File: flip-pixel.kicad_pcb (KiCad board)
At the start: 2 copper layers, 157.5 x 129.5 mm, 183 parts, among them J1 Barrel-Jack, Q1 DMN62D0U-7, Q10 STS8DN6LF6AG, Q11 DMN62D0U-7, Q12 DMN62D0U-7, Q13 STS8DN6LF6AG, Q14 DMN62D0U-7, Q15 DMN62D0U-7, Q16 STS8DN6LF6AG, Q17 DMN62D0U-7, Q18 DMN62D0U-7, Q19 STS8DN6LF6AG, Q2 DMN62D0U-7, Q20 DMN62D0U-7, Q21 DMN62D0U-7, Q22 STS8DN6LF6AG, Q23 DMN62D0U-7, Q24 DMN62D0U-7, Q25 STS8DN6LF6AG, Q26 DMN62D0U-7, Q27 DMN62D0U-7, Q28 STS8DN6LF6AG, Q29 DMN62D0U-7, Q3 DMN62D0U-7, Q30 DMN62D0U-7, Q31 STS8DN6LF6AG, Q4 STS8DN6LF6AG, Q5 DMN62D0U-7, Q6 DMN62D0U-7, Q7 STS8DN6LF6AG, Q8 DMN62D0U-7, Q9 DMN62D0U-7, U1 LM2665M6, U2 ESP32_DevBoard, U3 INA250A3

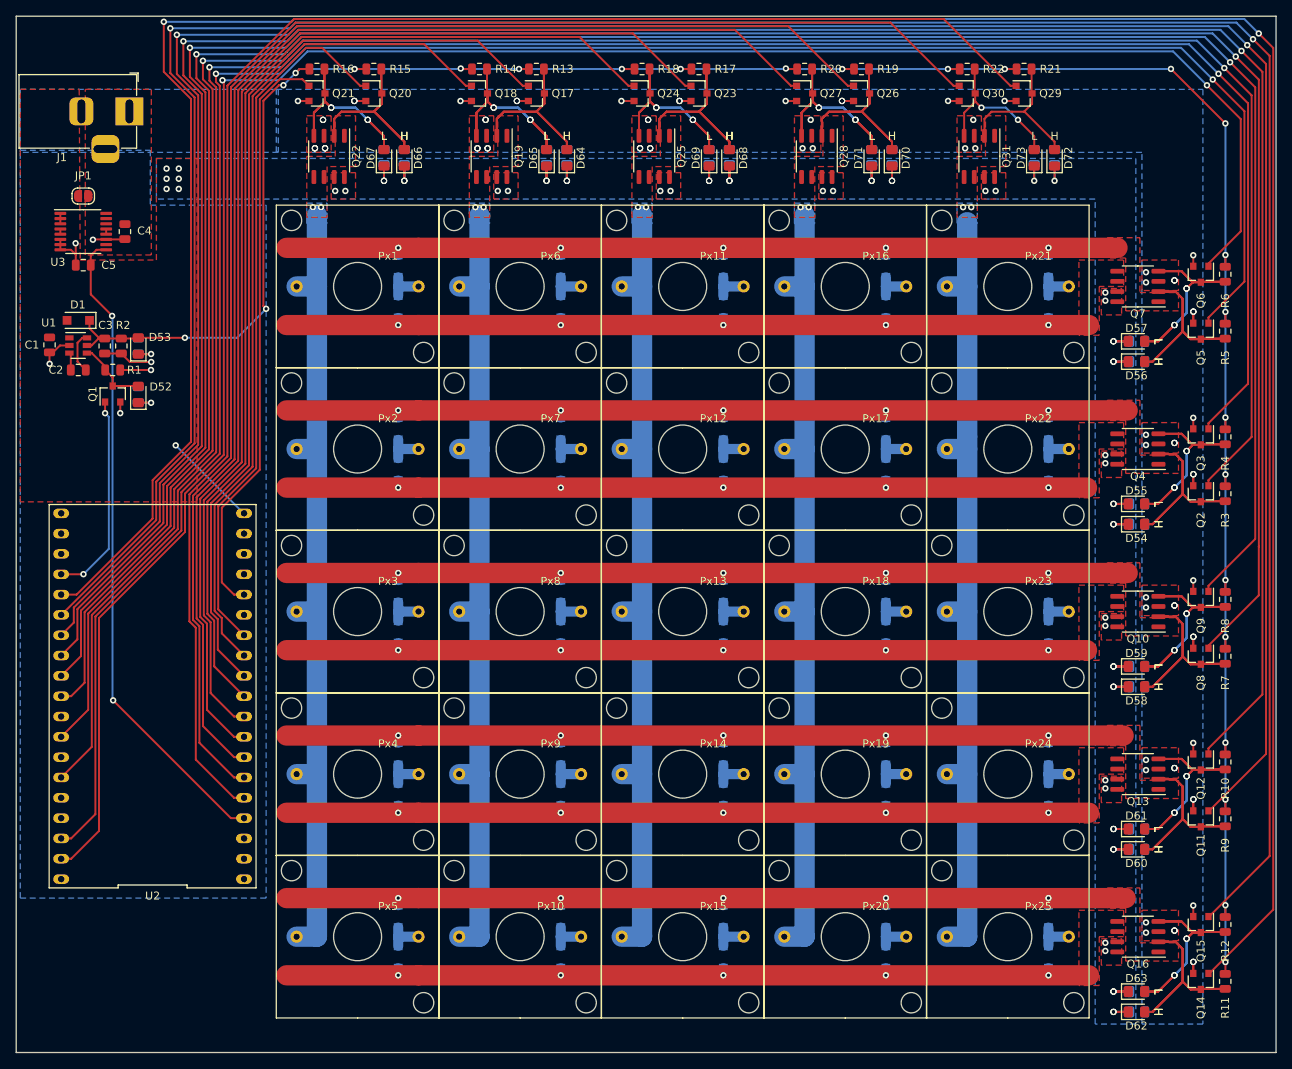
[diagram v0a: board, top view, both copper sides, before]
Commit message: Logos and SilkScreen
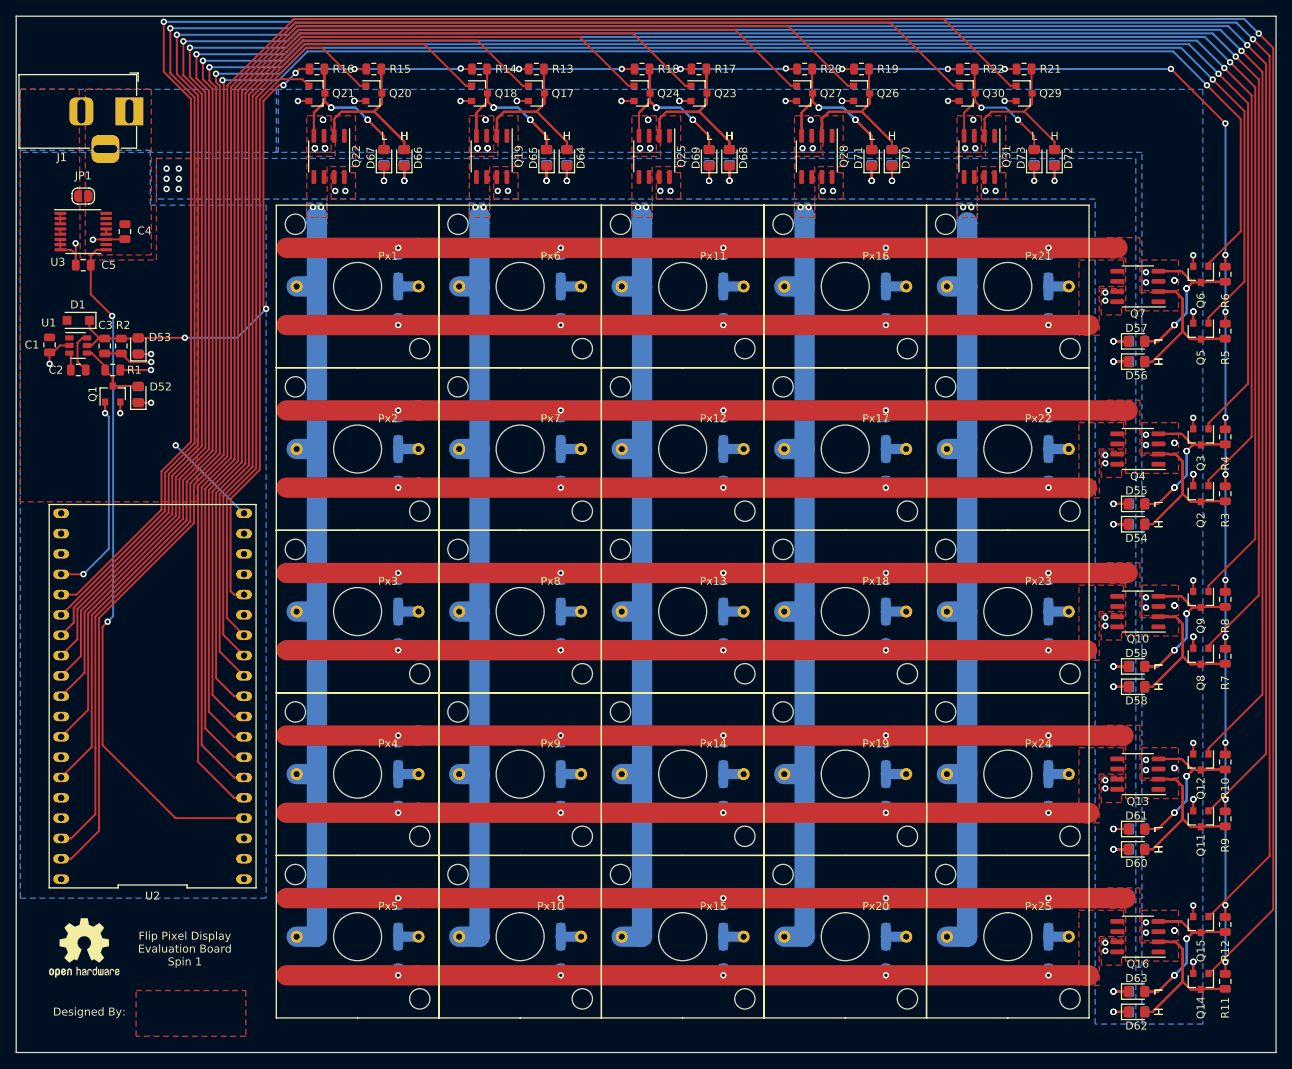
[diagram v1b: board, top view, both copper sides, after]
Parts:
- added LOGO1: Logo_Open_Hardware_Small, Symbol:OSHW-Logo2_9.8x8mm_SilkScreen, F.Cu at (62.1, 144.4)
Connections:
- D10 pad 1: Net-(D2-Pad1) -> Net-(D10-Pad1)
- D10 pad 2: /Row1/High -> /Row5/High
- D11 pad 1: /Row1/Low -> /Row5/Low
- D11 pad 2: Net-(D2-Pad1) -> Net-(D10-Pad1)
- D12 pad 1: Net-(D2-Pad1) -> Net-(D12-Pad1)
- D13 pad 2: Net-(D2-Pad1) -> Net-(D12-Pad1)
- D14 pad 1: Net-(D2-Pad1) -> Net-(D14-Pad1)
- D14 pad 2: /Row1/High -> /Row2/High
- D15 pad 1: /Row1/Low -> /Row2/Low
- D15 pad 2: Net-(D2-Pad1) -> Net-(D14-Pad1)
- D16 pad 1: Net-(D2-Pad1) -> Net-(D16-Pad1)
- D16 pad 2: /Row1/High -> /Row3/High
- D17 pad 1: /Row1/Low -> /Row3/Low
- D17 pad 2: Net-(D2-Pad1) -> Net-(D16-Pad1)
- D18 pad 1: Net-(D2-Pad1) -> Net-(D18-Pad1)
- D18 pad 2: /Row1/High -> /Row4/High
- D19 pad 1: /Row1/Low -> /Row4/Low
- D19 pad 2: Net-(D2-Pad1) -> Net-(D18-Pad1)
- D20 pad 1: Net-(D2-Pad1) -> Net-(D20-Pad1)
- D20 pad 2: /Row1/High -> /Row5/High
- D21 pad 1: /Row1/Low -> /Row5/Low
- D21 pad 2: Net-(D2-Pad1) -> Net-(D20-Pad1)
- D22 pad 1: Net-(D2-Pad1) -> Net-(D22-Pad1)
- D23 pad 2: Net-(D2-Pad1) -> Net-(D22-Pad1)
- D24 pad 1: Net-(D2-Pad1) -> Net-(D24-Pad1)
- D24 pad 2: /Row1/High -> /Row2/High
- D25 pad 1: /Row1/Low -> /Row2/Low
- D25 pad 2: Net-(D2-Pad1) -> Net-(D24-Pad1)
- D26 pad 1: Net-(D2-Pad1) -> Net-(D26-Pad1)
- D26 pad 2: /Row1/High -> /Row3/High
- D27 pad 1: /Row1/Low -> /Row3/Low
- D27 pad 2: Net-(D2-Pad1) -> Net-(D26-Pad1)
- D28 pad 1: Net-(D2-Pad1) -> Net-(D28-Pad1)
- D28 pad 2: /Row1/High -> /Row4/High
- D29 pad 1: /Row1/Low -> /Row4/Low
- D29 pad 2: Net-(D2-Pad1) -> Net-(D28-Pad1)
- D30 pad 1: Net-(D2-Pad1) -> Net-(D30-Pad1)
- D30 pad 2: /Row1/High -> /Row5/High
- D31 pad 1: /Row1/Low -> /Row5/Low
- D31 pad 2: Net-(D2-Pad1) -> Net-(D30-Pad1)
- D32 pad 1: Net-(D2-Pad1) -> Net-(D32-Pad1)
- D33 pad 2: Net-(D2-Pad1) -> Net-(D32-Pad1)
- D34 pad 1: Net-(D2-Pad1) -> Net-(D34-Pad1)
- D34 pad 2: /Row1/High -> /Row2/High
- D35 pad 1: /Row1/Low -> /Row2/Low
- D35 pad 2: Net-(D2-Pad1) -> Net-(D34-Pad1)
- D36 pad 1: Net-(D2-Pad1) -> Net-(D36-Pad1)
- D36 pad 2: /Row1/High -> /Row3/High
- D37 pad 1: /Row1/Low -> /Row3/Low
- D37 pad 2: Net-(D2-Pad1) -> Net-(D36-Pad1)
- D38 pad 1: Net-(D2-Pad1) -> Net-(D38-Pad1)
- D38 pad 2: /Row1/High -> /Row4/High
- D39 pad 1: /Row1/Low -> /Row4/Low
- D39 pad 2: Net-(D2-Pad1) -> Net-(D38-Pad1)
- D4 pad 1: Net-(D2-Pad1) -> Net-(D4-Pad1)
- D4 pad 2: /Row1/High -> /Row2/High
- D40 pad 1: Net-(D2-Pad1) -> Net-(D40-Pad1)
- D40 pad 2: /Row1/High -> /Row5/High
- D41 pad 1: /Row1/Low -> /Row5/Low
- D41 pad 2: Net-(D2-Pad1) -> Net-(D40-Pad1)
- D42 pad 1: Net-(D2-Pad1) -> Net-(D42-Pad1)
- D43 pad 2: Net-(D2-Pad1) -> Net-(D42-Pad1)
- D44 pad 1: Net-(D2-Pad1) -> Net-(D44-Pad1)
- D44 pad 2: /Row1/High -> /Row2/High
- D45 pad 1: /Row1/Low -> /Row2/Low
- D45 pad 2: Net-(D2-Pad1) -> Net-(D44-Pad1)
- D46 pad 1: Net-(D2-Pad1) -> Net-(D46-Pad1)
- D46 pad 2: /Row1/High -> /Row3/High
- D47 pad 1: /Row1/Low -> /Row3/Low
- D47 pad 2: Net-(D2-Pad1) -> Net-(D46-Pad1)
- D48 pad 1: Net-(D2-Pad1) -> Net-(D48-Pad1)
- D48 pad 2: /Row1/High -> /Row4/High
- D49 pad 1: /Row1/Low -> /Row4/Low
- D49 pad 2: Net-(D2-Pad1) -> Net-(D48-Pad1)
- D5 pad 1: /Row1/Low -> /Row2/Low
- D5 pad 2: Net-(D2-Pad1) -> Net-(D4-Pad1)
- D50 pad 1: Net-(D2-Pad1) -> Net-(D50-Pad1)
- D50 pad 2: /Row1/High -> /Row5/High
- D51 pad 1: /Row1/Low -> /Row5/Low
- D51 pad 2: Net-(D2-Pad1) -> Net-(D50-Pad1)
- D6 pad 1: Net-(D2-Pad1) -> Net-(D6-Pad1)
- D6 pad 2: /Row1/High -> /Row3/High
- D7 pad 1: /Row1/Low -> /Row3/Low
- D7 pad 2: Net-(D2-Pad1) -> Net-(D6-Pad1)
- D8 pad 1: Net-(D2-Pad1) -> Net-(D8-Pad1)
- D8 pad 2: /Row1/High -> /Row4/High
- D9 pad 1: /Row1/Low -> /Row4/Low
- D9 pad 2: Net-(D2-Pad1) -> Net-(D8-Pad1)
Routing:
- net /Row1/High: track 545.9 -> 108.3 mm, vias 25 -> 5
- net /Row1/Low: track 523.3 -> 104.8 mm, vias 25 -> 5
- net Net-(D2-Pad1): track 120.5 -> 4.82 mm
- net /Row2/High: track 0.00 -> 109.6 mm, vias 0 -> 5
- net /Row3/High: track 0.00 -> 109.6 mm, vias 0 -> 5
- net /Row5/High: track 0.00 -> 109.3 mm, vias 0 -> 5
- net /Row4/High: track 0.00 -> 109.1 mm, vias 0 -> 5
- net /Row5/Low: track 0.00 -> 104.8 mm, vias 0 -> 5
- net /Row4/Low: track 0.00 -> 104.8 mm, vias 0 -> 5
- net /Row3/Low: track 0.00 -> 104.5 mm, vias 0 -> 5
- net /Row2/Low: track 0.00 -> 104.5 mm, vias 0 -> 5
- net /current: track 81.4 -> 86.6 mm
- net Net-(D30-Pad1): track 0.00 -> 4.82 mm
- net Net-(D28-Pad1): track 0.00 -> 4.82 mm
- net Net-(D26-Pad1): track 0.00 -> 4.82 mm
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- added copper zone on F.Cu, net (none)
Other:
- board text added: "Connor Winiarczyk"
- board text added: "Designed By:"
- board text added: "Flip Pixel Display Evaluation Board Spin 1"
- board text added: "https://github.com/Hayden-and-Connor/flip-pixel"
